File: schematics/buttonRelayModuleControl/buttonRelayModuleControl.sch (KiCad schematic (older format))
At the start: 18 parts, among them J1 Conn_AC_MAINS, J2 Programmer, SW1 SW_Push_LED, SW2 SW_Push_LED, U2 TSP-05, U3 ATmega328PB-AU

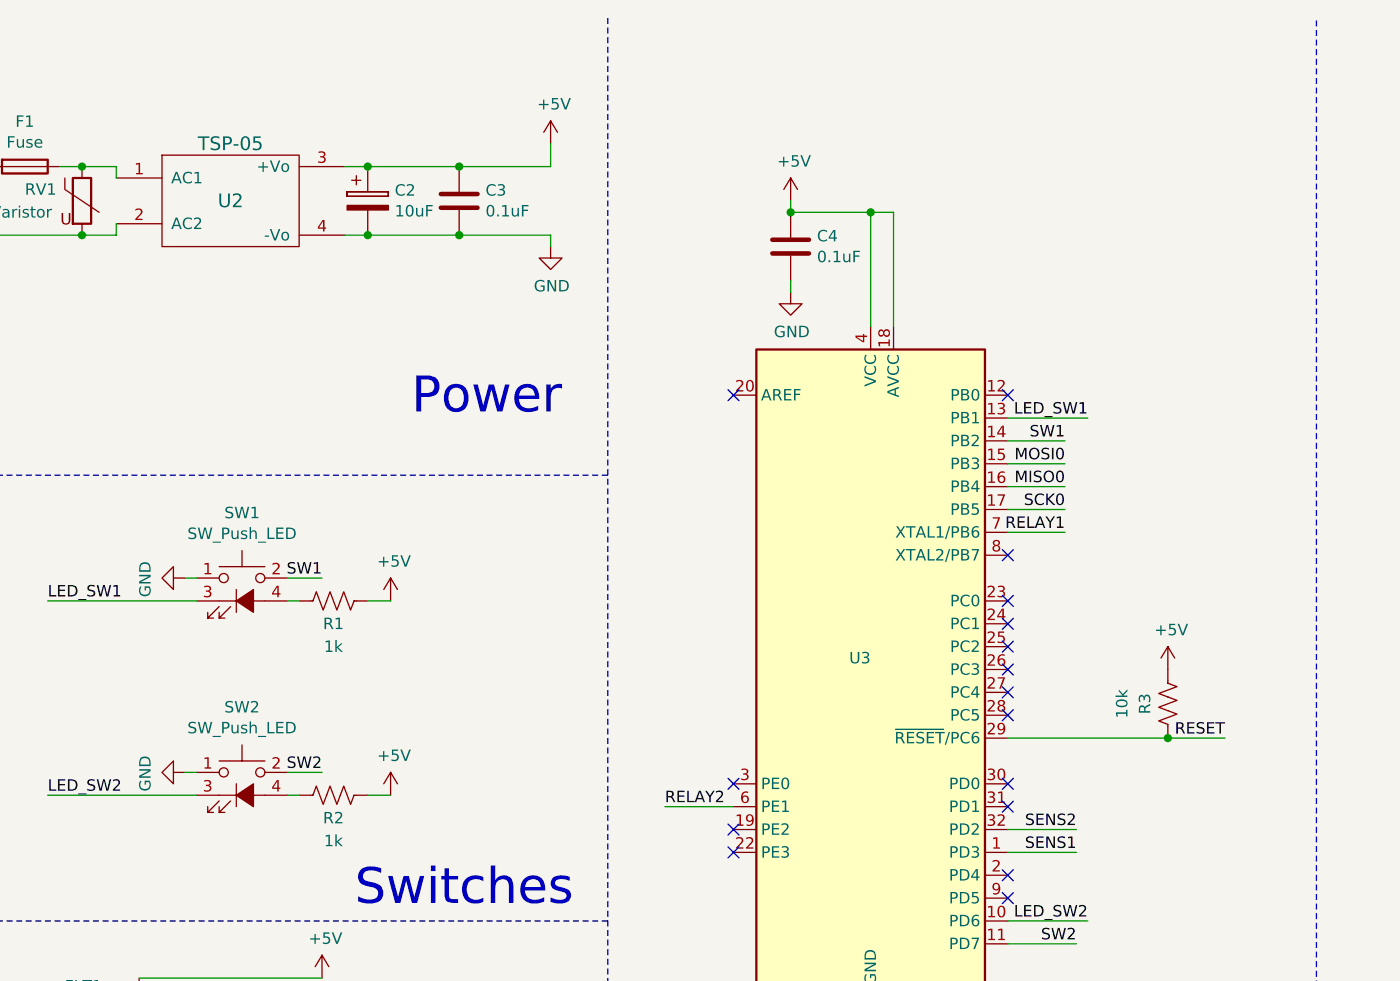
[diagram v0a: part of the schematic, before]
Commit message: Initial Firmware
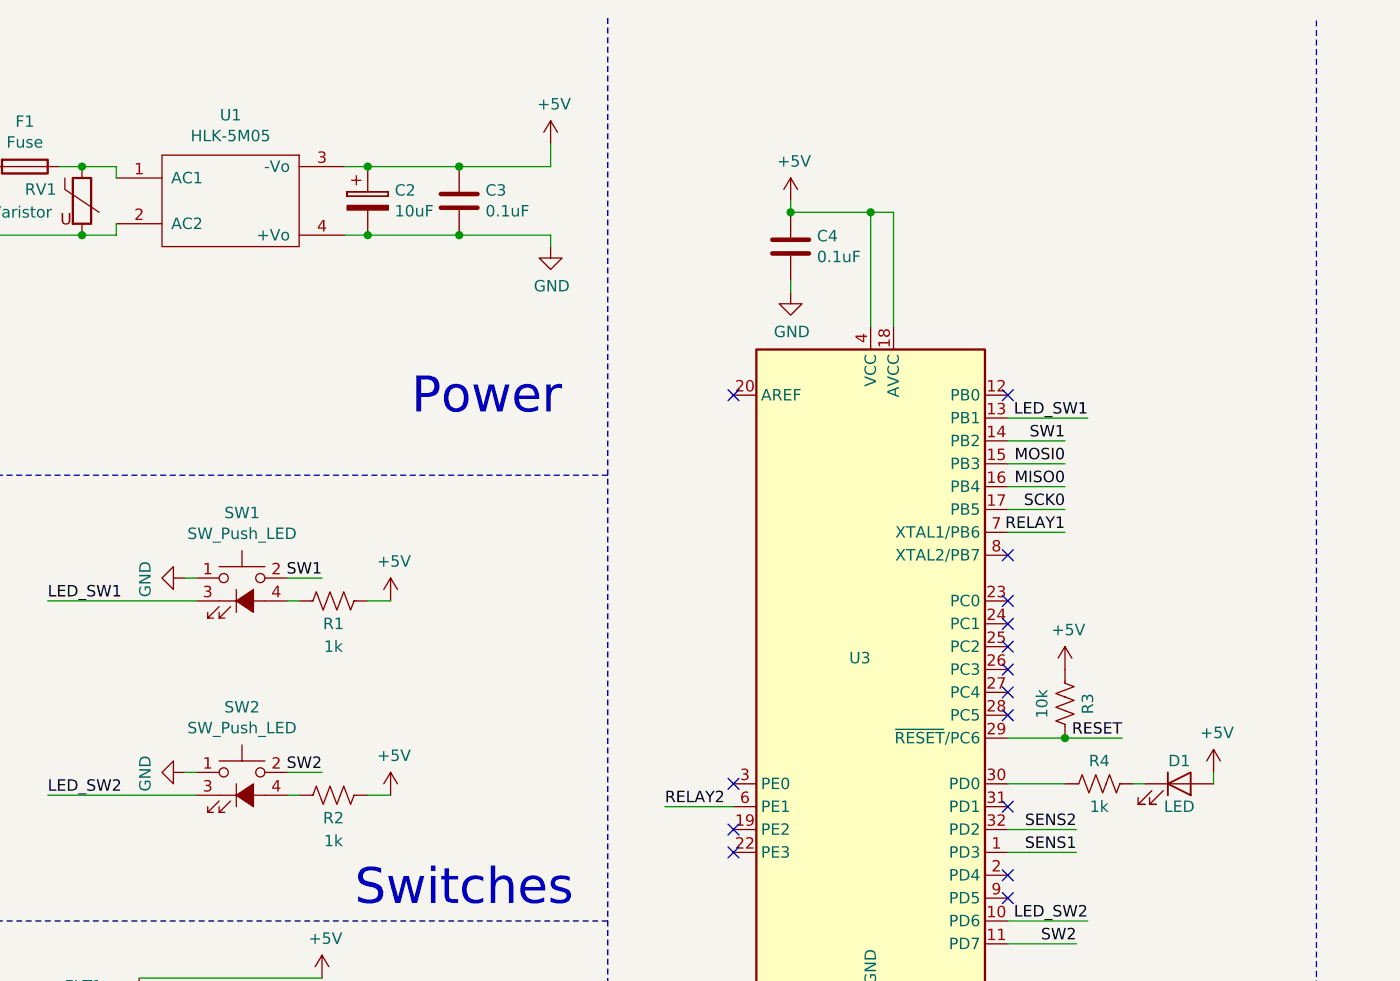
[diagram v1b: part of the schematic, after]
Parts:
- removed U2: TSP-05, Power_Supply:HLK-PM05, symbol remoteSwitch_custom:TSP-03
- added D1: LED, LED_SMD:LED_0603_1608Metric_Pad1.05x0.95mm_HandSolder, symbol Device:LED
- added R4: 1k, Resistor_SMD:R_0805_2012Metric_Pad1.15x1.40mm_HandSolder, symbol Device:R_US
- added U1: HLK-5M05, remoteSwitch_footprints:HLK-5M05, symbol remoteSwitch_custom:HLK-5M05
- FLT1, FLT2: footprint Connectors_JST:JST_PH_B4B-PH-K_1x04_P2.00mm_Vertical -> Connector_JST:JST_XH_B04B-XH-A_1x04_P2.50mm_Vertical
- RLY1, RLY2: footprint Connector_PinHeader_2.54mm:PinHeader_1x03_P2.54mm_Vertical -> Connector_JST:JST_XH_B03B-XH-A_1x03_P2.50mm_Vertical
- SW1, SW2: footprint Connector_PinHeader_2.54mm:PinHeader_1x04_P2.54mm_Vertical -> Connector_JST:JST_XH_B04B-XH-A_1x04_P2.50mm_Vertical
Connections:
- wire segments 67 -> 70
- no-connect marks 16 -> 15
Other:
- moved on the sheet: R3
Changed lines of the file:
@@
 $EndDescr
-$Comp
-L remoteSwitch_custom:TSP-03 U2
-U 1 1 5B5E5DB0
-P 2200 1300
-F 0 "U2" H 2200 1300 60  0000 C CNN
-F 1 "TSP-05" H 2200 1550 60  0000 C CNN
-F 2 "Power_Supply:HLK-PM05" H 2200 1300 60  0001 C CNN
-F 3 "" H 2200 1300 60  0000 C CNN
-	1    2200 1300
-	1    0    0    -1
-$EndComp
 $Comp
 L Connector:Screw_Terminal_01x02 J1
@@
 F 0 "SW1" H 2250 3435 50  0000 C CNN
 F 1 "SW_Push_LED" H 2250 3344 50  0000 C CNN
-F 2 "Connector_PinHeader_2.54mm:PinHeader_1x04_P2.54mm_Vertical" H 2250 3350 50  0001 C CNN
+F 2 "Connector_JST:JST_XH_B04B-XH-A_1x04_P2.50mm_Vertical" H 2250 3350 50  0001 C CNN
 F 3 "" H 2250 3350 50  0001 C CNN
 	1    2250 3050
@@
 F 0 "SW2" H 2250 4285 50  0000 C CNN
 F 1 "SW_Push_LED" H 2250 4194 50  0000 C CNN
-F 2 "Connector_PinHeader_2.54mm:PinHeader_1x04_P2.54mm_Vertical" H 2250 4200 50  0001 C CNN
+F 2 "Connector_JST:JST_XH_B04B-XH-A_1x04_P2.50mm_Vertical" H 2250 4200 50  0001 C CNN
 F 3 "" H 2250 4200 50  0001 C CNN
 	1    2250 3900
@@
 L Device:R_US R3
 U 1 1 5B605473
-P 6300 3500
-F 0 "R3" V 6400 3500 50  0000 C CNN
-F 1 "10k" V 6500 3500 50  0000 C CNN
-F 2 "Resistor_SMD:R_1206_3216Metric_Pad1.42x1.75mm_HandSolder" V 6340 3490 50  0001 C CNN
-F 3 "~" H 6300 3500 50  0001 C CNN
-	1    6300 3500
+P 5850 3500
+F 0 "R3" V 5750 3500 50  0000 C CNN
+F 1 "10k" V 5950 3500 50  0000 C CNN
+F 2 "Resistor_SMD:R_1206_3216Metric_Pad1.42x1.75mm_HandSolder" V 5890 3490 50  0001 C CNN
+F 3 "~" H 5850 3500 50  0001 C CNN
+	1    5850 3500
 	-1   0    0    1
 $EndComp
@@
 Wire Wire Line
 	5600 2650 5850 2650
-Wire Wire Line
-	6300 3650 5600 3650
-Connection ~ 6300 3650
 $Comp
 L power:GND #PWR0115
@@
 Text Label 5900 4550 2    50   ~ 0
 SW2
-Text Label 6550 3650 2    50   ~ 0
+Text Label 6100 3650 2    50   ~ 0
 RESET
 Text Label 5850 2450 2    50   ~ 0
@@
 LED_SW2
 Wire Wire Line
-	6300 3650 6550 3650
+	5850 3650 6100 3650
 Wire Wire Line
 	7650 2300 7950 2300
 Text Label 5850 2350 2    50   ~ 0
 SW1
-NoConn ~ 5600 3850
 NoConn ~ 5600 3950
 NoConn ~ 5600 3050
@@
 F 0 "FLT1" H 1556 5665 50  0000 C CNN
 F 1 "FLOAT" H 1556 5574 50  0000 C CNN
-F 2 "Connectors_JST:JST_PH_B4B-PH-K_1x04_P2.00mm_Vertical" H 1500 5195 50  0001 C CNN
+F 2 "Connector_JST:JST_XH_B04B-XH-A_1x04_P2.50mm_Vertical" H 1500 5195 50  0001 C CNN
 F 3 "" H 1500 5195 50  0001 C CNN
 	1    1350 5200
@@
 L power:+5V #PWR010
 U 1 1 5BD3D829
-P 6300 3350
-F 0 "#PWR010" H 6300 3200 50  0001 C CNN
-F 1 "+5V" H 6315 3523 50  0000 C CNN
-F 2 "" H 6300 3350 50  0001 C CNN
-F 3 "" H 6300 3350 50  0001 C CNN
-	1    6300 3350
+P 5850 3350
+F 0 "#PWR010" H 5850 3200 50  0001 C CNN
+F 1 "+5V" H 5865 3523 50  0000 C CNN
+F 2 "" H 5850 3350 50  0001 C CNN
+F 3 "" H 5850 3350 50  0001 C CNN
+	1    5850 3350
 	1    0    0    -1
 $EndComp
@@
 F 0 "RLY2" H 8828 2346 50  0000 L CNN
 F 1 "RELAY" H 8828 2255 50  0000 L CNN
-F 2 "Connector_PinHeader_2.54mm:PinHeader_1x03_P2.54mm_Vertical" H 8550 2300 50  0001 C CNN
+F 2 "Connector_JST:JST_XH_B03B-XH-A_1x03_P2.50mm_Vertical" H 8550 2300 50  0001 C CNN
 F 3 "" H 8550 2300 50  0001 C CNN
 	1    8450 2300
@@
 F 0 "RLY1" H 8828 3946 50  0000 L CNN
 F 1 "RELAY" H 8828 3855 50  0000 L CNN
-F 2 "Connector_PinHeader_2.54mm:PinHeader_1x03_P2.54mm_Vertical" H 8550 3900 50  0001 C CNN
+F 2 "Connector_JST:JST_XH_B03B-XH-A_1x03_P2.50mm_Vertical" H 8550 3900 50  0001 C CNN
 F 3 "" H 8550 3900 50  0001 C CNN
 	1    8450 3900
@@
 F 0 "FLT2" H 1856 7065 50  0000 C CNN
 F 1 "FLOAT" H 1856 6974 50  0000 C CNN
-F 2 "Connectors_JST:JST_PH_B4B-PH-K_1x04_P2.00mm_Vertical" H 1800 6595 50  0001 C CNN
+F 2 "Connector_JST:JST_XH_B04B-XH-A_1x04_P2.50mm_Vertical" H 1800 6595 50  0001 C CNN
 F 3 "" H 1800 6595 50  0001 C CNN
 	1    1650 6600
@@
 	5600 4550 5900 4550
 NoConn ~ 5600 3250
+$Comp
+L remoteSwitch_custom:HLK-5M05 U1
+U 1 1 5BCD3DE1
+P 2200 1300
+F 0 "U1" H 2200 1675 50  0000 C CNN
+F 1 "HLK-5M05" H 2200 1584 50  0000 C CNN
+F 2 "remoteSwitch_footprints:HLK-5M05" H 2200 1300 50  0001 C CNN
+F 3 "" H 2200 1300 50  0001 C CNN
+	1    2200 1300
+	1    0    0    -1
+$EndComp
+Wire Wire Line
+	5600 3650 5850 3650
+Connection ~ 5850 3650
+$Comp
+L Device:R_US R4
+U 1 1 5BCD4302
+P 6000 3850
+F 0 "R4" V 5900 3850 50  0000 C CNN
+F 1 "1k" V 6100 3850 50  0000 C CNN
+F 2 "Resistor_SMD:R_0805_2012Metric_Pad1.15x1.40mm_HandSolder" V 6040 3840 50  0001 C CNN
+F 3 "~" H 6000 3850 50  0001 C CNN
+	1    6000 3850
+	0    1    1    0
+$EndComp
+$Comp
+L Device:LED D1
+U 1 1 5BCD443C
+P 6350 3850
+F 0 "D1" H 6350 3950 50  0000 C CNN
+F 1 "LED" H 6350 3750 50  0000 C CNN
+F 2 "LED_SMD:LED_0603_1608Metric_Pad1.05x0.95mm_HandSolder" H 6350 3850 50  0001 C CNN
+F 3 "~" H 6350 3850 50  0001 C CNN
+	1    6350 3850
+	1    0    0    -1
+$EndComp
+$Comp
+L power:+5V #PWR015
+U 1 1 5BCD4490
+P 6500 3800
+F 0 "#PWR015" H 6500 3650 50  0001 C CNN
+F 1 "+5V" H 6515 3973 50  0000 C CNN
+F 2 "" H 6500 3800 50  0001 C CNN
+F 3 "" H 6500 3800 50  0001 C CNN
+	1    6500 3800
+	1    0    0    -1
+$EndComp
+Wire Wire Line
+	5600 3850 5850 3850
+Wire Wire Line
+	6150 3850 6200 3850
+Wire Wire Line
+	6500 3850 6500 3800
 $EndSCHEMATC
